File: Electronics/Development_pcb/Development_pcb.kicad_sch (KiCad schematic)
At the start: 15 parts, among them J1 TF-Luna, J2 Pan, J3 Tilt, J4 MP3, J5 Display, J6 LAZER, J7 CAM-PWR, J8 USB-C, Q1 2N2222A, U1 ESP32-S3-DEVKIT:C-1-N16R8, U2 MP3-TF-16P

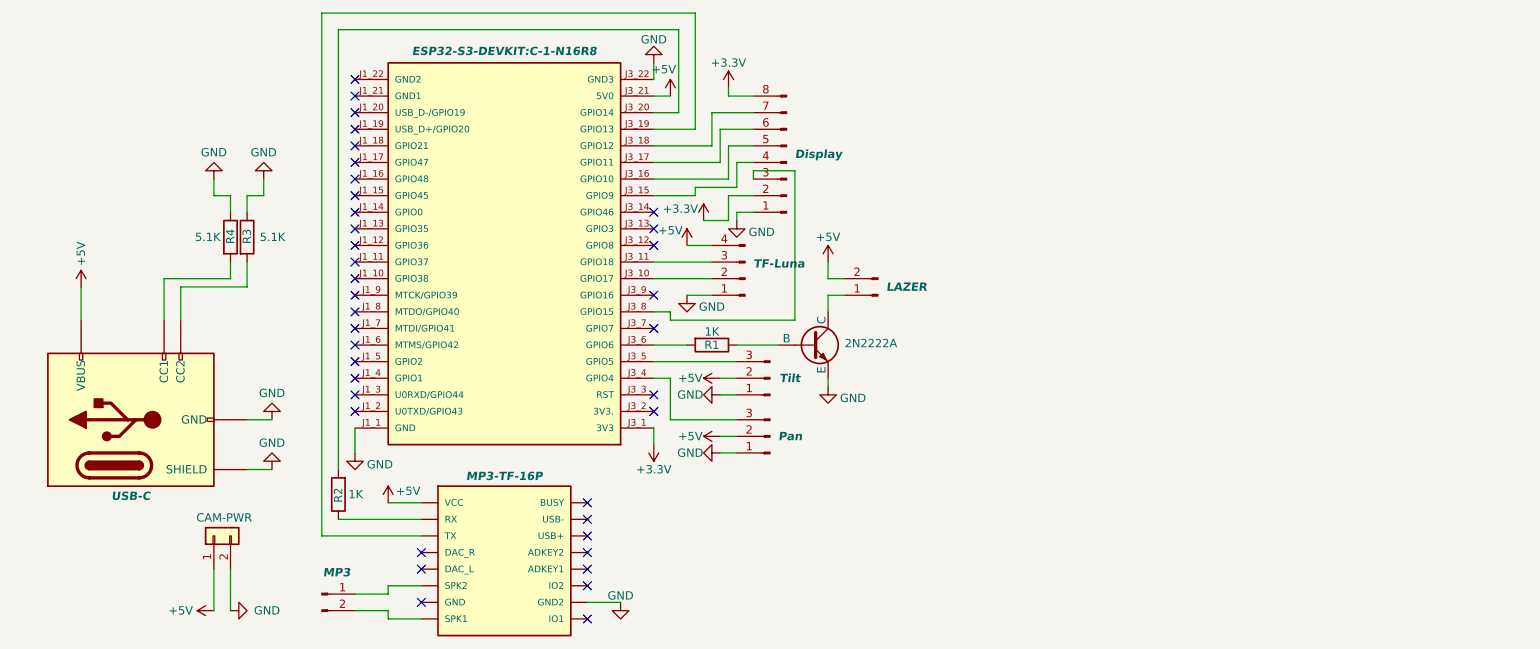
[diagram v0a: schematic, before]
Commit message: changes
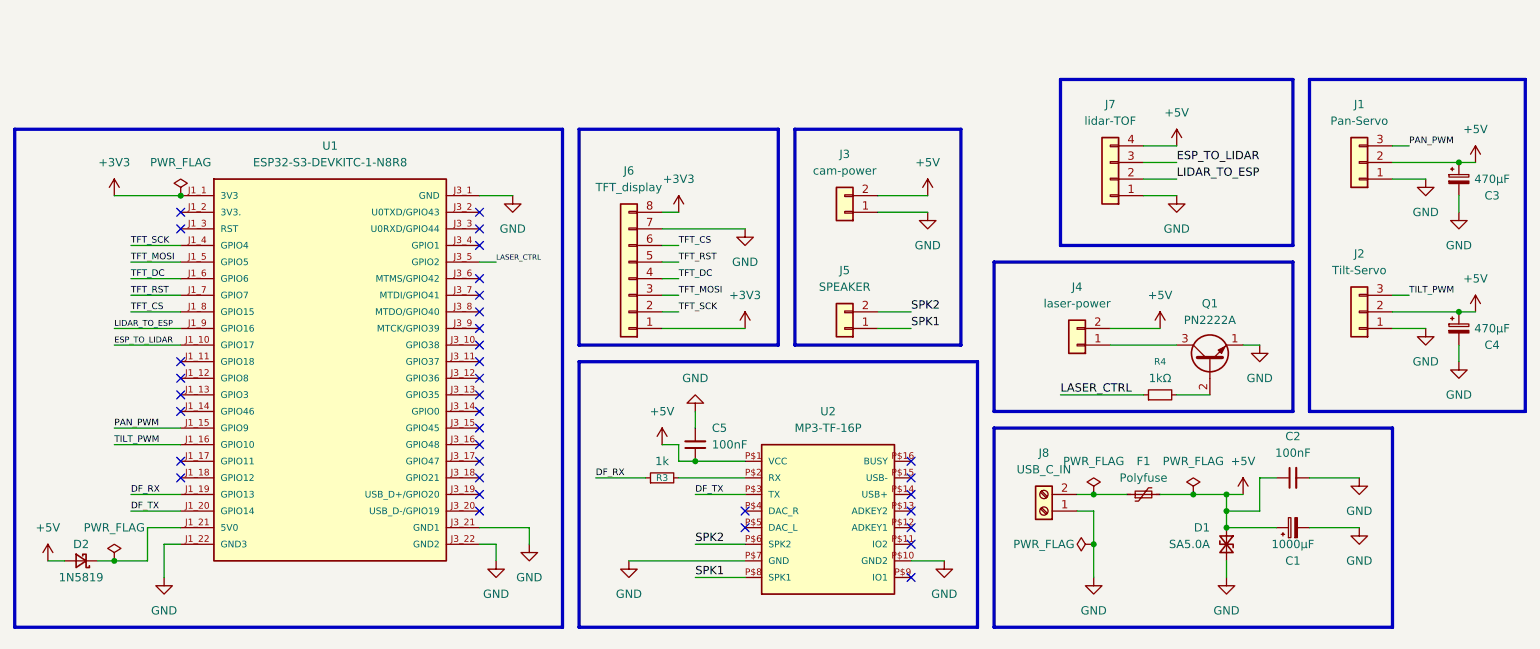
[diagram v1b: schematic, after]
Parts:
- removed J1: TF-Luna, Connector_PinHeader_2.54mm:PinHeader_1x04_P2.54mm_Vertical, symbol Connector:Conn_01x04_Pin
- removed J2: Pan, Connector_PinHeader_2.54mm:PinHeader_1x03_P2.54mm_Vertical, symbol Connector:Conn_01x03_Pin
- removed J3: Tilt, Connector_PinHeader_2.54mm:PinHeader_1x03_P2.54mm_Vertical, symbol Connector:Conn_01x03_Pin
- removed J4: MP3, Connector_PinHeader_2.54mm:PinHeader_1x02_P2.54mm_Vertical, symbol Connector:Conn_01x02_Pin
- removed J5: Display, Connector_PinHeader_2.54mm:PinHeader_1x08_P2.54mm_Vertical, symbol Connector:Conn_01x08_Pin
- removed J6: LAZER, Connector_PinHeader_2.54mm:PinHeader_1x02_P2.54mm_Vertical, symbol Connector:Conn_01x02_Pin
- removed J7: CAM-PWR, Connector_PinHeader_2.54mm:PinHeader_1x02_P2.54mm_Vertical, symbol Connector_Generic:Conn_01x02
- removed J8: USB-C, Connector_USB:USB_C_Receptacle_HRO_TYPE-C-31-M-12, symbol Connector:USB_C_Receptacle_PowerOnly_6P
- removed Q1: 2N2222A, Package_TO_SOT_THT:TO-92_Inline, symbol Simulation_SPICE:NPN
- removed R1, R2: 1K, Resistor_THT:R_Axial_DIN0207_L6.3mm_D2.5mm_P7.62mm_Horizontal, symbol Device:R
- removed R3, R4: 5.1K, Resistor_THT:R_Axial_DIN0207_L6.3mm_D2.5mm_P7.62mm_Horizontal, symbol Device:R
- added C1: 1000µF, Capacitor_THT:CP_Radial_D10.0mm_P5.00mm, symbol Device:C_Polarized_Small
- added C2, C5: 100nF, Capacitor_THT:C_Disc_D5.0mm_W2.5mm_P5.00mm, symbol Device:C_Small
- added C3, C4: 470µF, Capacitor_THT:CP_Radial_D8.0mm_P3.50mm, symbol Device:C_Polarized_Small
- added D1: SA5.0A, Diode_THT:D_DO-15_P10.16mm_Horizontal, symbol Device:D_TVS_Small
- added D2: 1N5819, Diode_THT:D_DO-41_SOD81_P10.16mm_Horizontal, symbol Device:D_Schottky_Small
- added F1: Polyfuse, Capacitor_THT:C_Disc_D5.0mm_W2.5mm_P5.00mm, symbol Device:Polyfuse_Small
- added J1: Pan-Servo, Connector_PinHeader_2.54mm:PinHeader_1x03_P2.54mm_Vertical, symbol Connector_Generic:Conn_01x03
- added J2: Tilt-Servo, Connector_PinHeader_2.54mm:PinHeader_1x03_P2.54mm_Vertical, symbol Connector_Generic:Conn_01x03
- added J3: cam-power, Connector_JST:JST_XH_B2B-XH-A_1x02_P2.50mm_Vertical, symbol Connector_Generic:Conn_01x02
- added J4: laser-power, Connector_JST:JST_XH_B2B-XH-A_1x02_P2.50mm_Vertical, symbol Connector_Generic:Conn_01x02
- added J5: SPEAKER, Connector_JST:JST_XH_B2B-XH-A_1x02_P2.50mm_Vertical, symbol Connector_Generic:Conn_01x02
- added J6: TFT_display, Connector_JST:JST_XH_B8B-XH-A_1x08_P2.50mm_Vertical, symbol Connector_Generic:Conn_01x08
- added J7: lidar-TOF, Connector_PinHeader_2.54mm:PinHeader_1x04_P2.54mm_Vertical, symbol Connector_Generic:Conn_01x04
- added J8: USB_C_IN, TerminalBlock_Phoenix:TerminalBlock_Phoenix_MKDS-3-2-5.08_1x02_P5.08mm_Horizontal, symbol Connector:Screw_Terminal_01x02
- added Q1: PN2222A, Package_TO_SOT_THT:TO-92_Inline, symbol Transistor_BJT:Q_NPN_EBC
- added R3: 1k, Resistor_THT:R_Axial_DIN0207_L6.3mm_D2.5mm_P10.16mm_Horizontal, symbol Device:R_Small
- added R4: 1kΩ, Resistor_THT:R_Axial_DIN0207_L6.3mm_D2.5mm_P10.16mm_Horizontal, symbol Device:R_Small
- U1: value ESP32-S3-DEVKIT:C-1-N16R8 -> ESP32-S3-DEVKITC-1-N8R8; footprint ESP32-S3-DEVKITC-1-N8R8:ESP32-S3-DEVKITC-1-N8R8 -> Development_pcb:ESP32-S3-DevKitC-1_Socket; Description_1 The ESP32-S3-DEVKITC-1-N8R8 from Espressif Systems is a dev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 -> (none)
- U2: Description_1 MP3 player module data sheet -> (none)
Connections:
- net +3.3V is gone; now on net GND: U1.J3_1 (GND)
- net +5V: now also C1.1, C2.1, C3.1, C4.1, C5.1, D1.1 (A1), D2.2 (A), F1.2, J1.2 (Pin_2), J2.2 (Pin_2), J3.2 (Pin_2), J4.2 (Pin_2), J7.4 (Pin_4); no longer U1.J3_21 (5V0)
- net GND: now also U1.J1_22 (GND3), U1.J3_21 (GND1), U2.P$7 (GND), C1.2, C2.2, C3.2, C4.2, C5.2, D1.2 (A2), J1.1 (Pin_1), J2.1 (Pin_1), J3.1 (Pin_1), J6.7 (Pin_7), J7.1 (Pin_1), J8.1 (Pin_1), Q1.1 (E); no longer U1.J1_1 (GND)
- net SPK2: now reaches U2.P$6 (SPK2)
- net SPK2: now also J5.2 (Pin_2)
- net SPK1: now reaches U2.P$8 (SPK1)
- net SPK1: now also J5.1 (Pin_1)
- net at U2.P$2 (RX): now also R3.2
- net at U1.J3_19 (USB_D+/GPIO20): no longer U2.P$3 (TX)
- net ESP_TO_LIDAR: now reaches U1.J1_10 (GPIO17)
- net ESP_TO_LIDAR: now also J7.3 (Pin_3)
- net PAN_PWM: now reaches U1.J1_15 (GPIO9)
- net PAN_PWM: now also J1.3 (Pin_3)
- net TILT_PWM: now reaches U1.J1_16 (GPIO10)
- net TILT_PWM: now also J2.3 (Pin_3)
- net DF_RX: now reaches U1.J1_19 (GPIO13)
- net DF_RX: now also R3.1
- net DF_TX: now reaches U1.J1_20 (GPIO14)
- net DF_TX: now also U2.P$3 (TX)
- net at U1.J1_21 (5V0): now also D2.1 (K)
- net TFT_SCK: now reaches U1.J1_4 (GPIO4)
- net TFT_SCK: now also J6.2 (Pin_2)
- net TFT_MOSI: now reaches U1.J1_5 (GPIO5)
- net TFT_MOSI: now also J6.3 (Pin_3)
- net TFT_DC: now reaches U1.J1_6 (GPIO6)
- net TFT_DC: now also J6.4 (Pin_4)
- net TFT_RST: now reaches U1.J1_7 (GPIO7)
- net TFT_RST: now also J6.5 (Pin_5)
- net TFT_CS: now reaches U1.J1_8 (GPIO15)
- net TFT_CS: now also J6.6 (Pin_6)
- net LIDAR_TO_ESP: now reaches U1.J1_9 (GPIO16)
- net LIDAR_TO_ESP: now also J7.2 (Pin_2)
- net LASER_CTRL: now reaches U1.J3_5 (GPIO2)
- net LASER_CTRL: now also R4.1
- new net: Q1.2 (B), R4.2
- new net: F1.1, J8.2 (Pin_2)
- new net: J4.1 (Pin_1), Q1.3 (C)
- new net +3V3: J6.1 (Pin_1), J6.8 (Pin_8), U1.J1_1 (3V3)
- no-connect marks 38 -> 35
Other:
- title: MISA_PCB -> MISA-PCB
